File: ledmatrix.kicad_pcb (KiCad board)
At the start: 2 copper layers, 75.6 x 37.8 mm, 32 parts, among them J1 BUS_IN1, J2 BUS_IN2, J3 BUS_OUT1, J4 BUS_OUT2, Q1 PMV50XP, Q2 PMV50XP, Q3 PMV50XP, Q4 PMV50XP, Q5 PMV50XP, Q6 PMV50XP, Q7 PMV50XP, Q8 PMV50XP, U1 1588BS, U2 STP08DP05, U3 1588BS, U4 STP08DP05, U5 74HC138

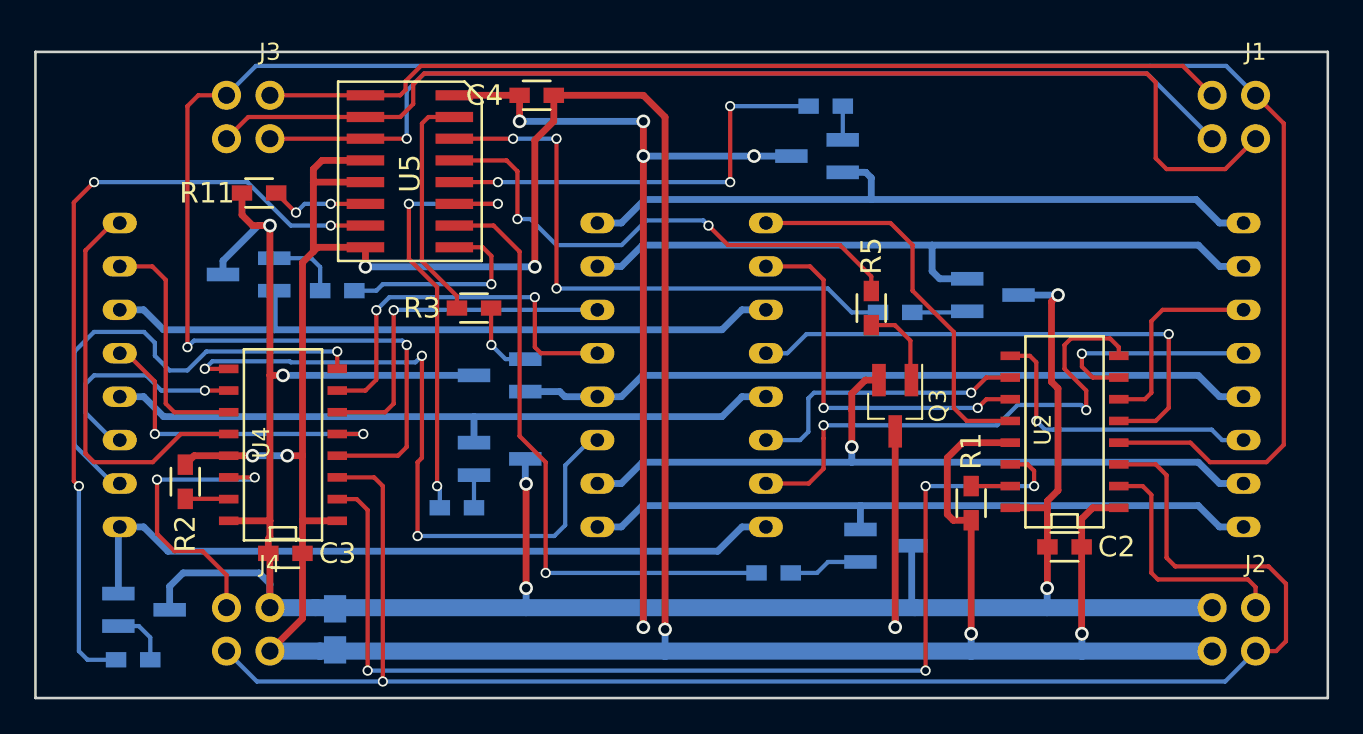
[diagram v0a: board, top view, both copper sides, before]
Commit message: generale gerbers
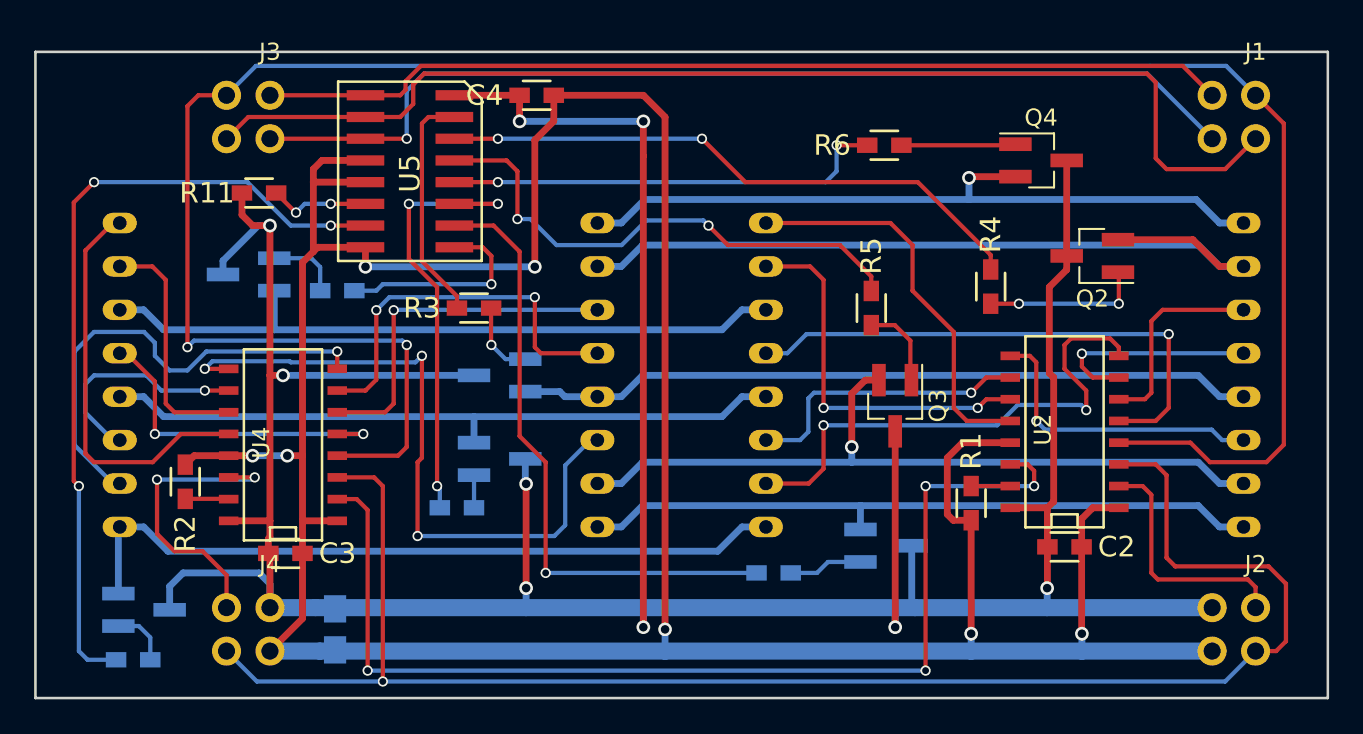
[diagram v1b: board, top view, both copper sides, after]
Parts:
- Q2, Q4, R4, R6: moved to F.Cu
- moved Q4 13.1 mm to (84.2, 31.8), turned to 0 degrees
- moved Q2 6.25 mm to (87.2, 37.3), turned to 180 degrees
- moved R4 5.79 mm to (81.3, 39.1), turned to 90 degrees
- moved R6 4.12 mm to (75.1, 30.9)
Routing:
- net Net-(Q2-Pad1): track 3.24 -> 9.40 mm, vias 0 -> 2
- net Net-(Q4-Pad1): track 1.97 -> 6.69 mm
- net /ROW_2: track 42.6 -> 46.9 mm
- net /VCC: track 210.5 -> 207.5 mm, vias 12 -> 9
- net /ROW_4: track 42.4 -> 43.4 mm, vias 0 -> 1
- net /Row Control/RC2: track 34.1 -> 35.0 mm, vias 3 -> 2
- net /Row Control/RC4: track 25.2 -> 25.9 mm, vias 3 -> 2
